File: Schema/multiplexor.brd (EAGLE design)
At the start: 100 x 80 mm, 23 parts, among them IC1 4051D, IC2 4051D, IC3 74LS595N

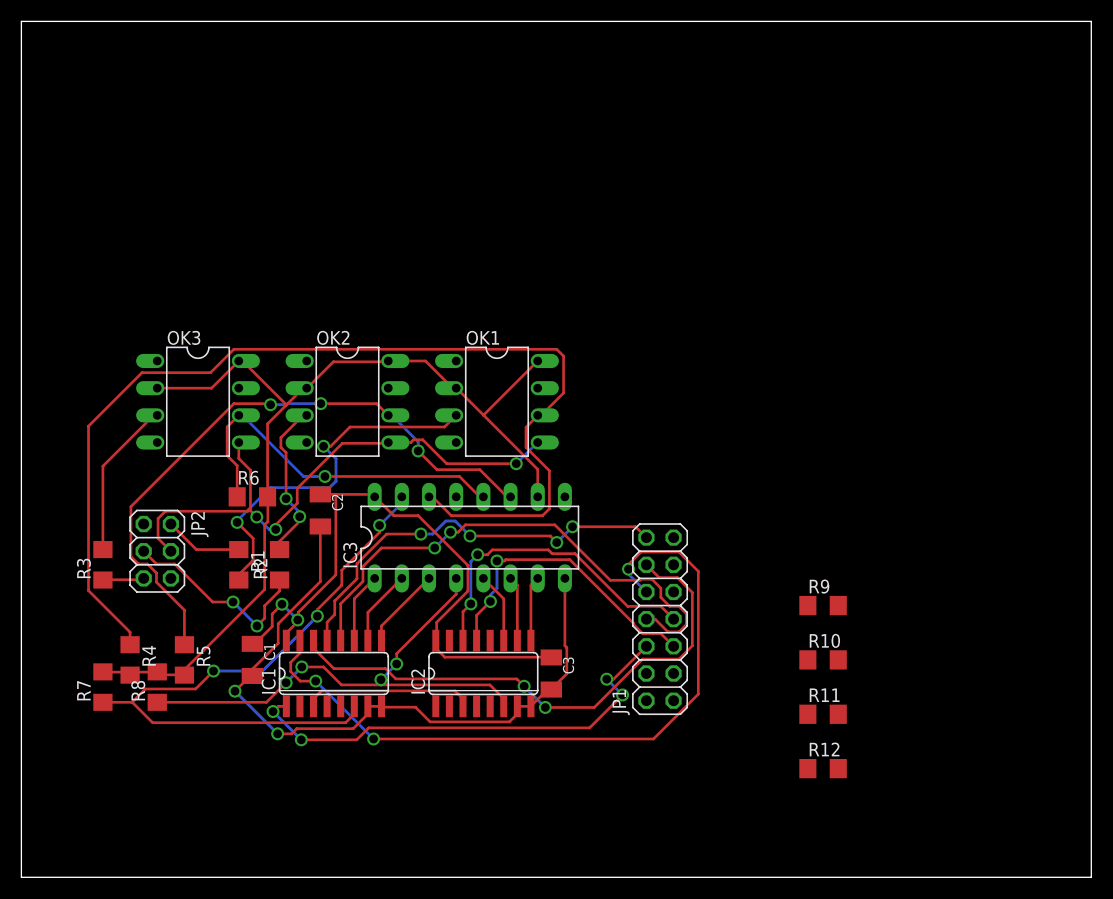
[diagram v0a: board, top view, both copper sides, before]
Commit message: Next release
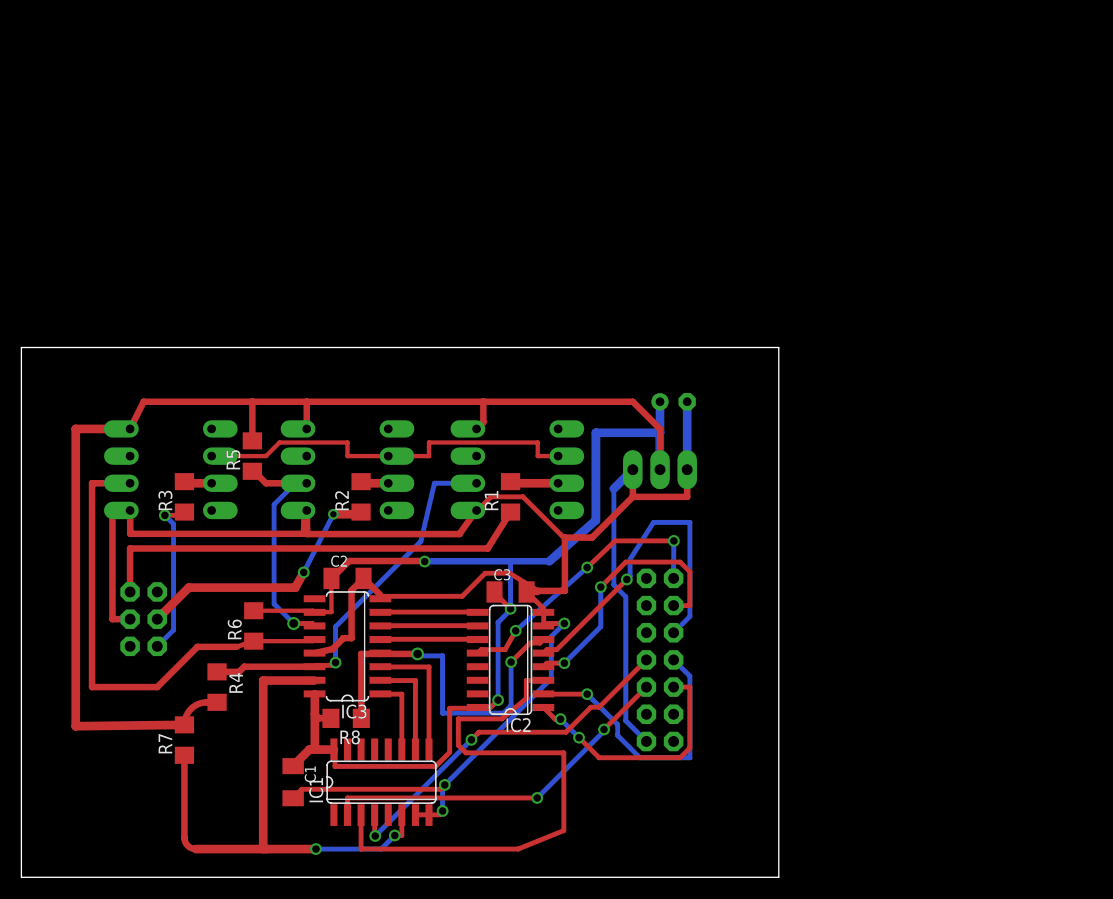
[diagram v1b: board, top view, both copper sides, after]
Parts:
- removed R10, R11, R12, R9: (no value), resistor:R1206
- added C4: (no value), rcl:E2,5-6
- added JP3: (no value), pinhead:1X03
- IC3: value 74LS595N -> 74HC595D; device 74xx-eu:DIL16 -> 74xx-eu:SO16
- moved R1 26.2 mm to (45.7, 35.6), turned to 90 degrees
- moved R5 20.1 mm to (21.6, 39.4), turned to 90 degrees
- moved R8 17.9 mm to (30.4, 14.9), turned to 180 degrees
- moved IC3 15.3 mm to (30.5, 21.6), turned to 90 degrees
- moved R6 12.1 mm to (21.7, 23.5), turned to 90 degrees
- moved C1 12.0 mm to (25.4, 8.89)
- moved IC1 11.1 mm to (33.7, 8.89)
- moved R2 9.92 mm to (31.8, 35.6)
- moved R3 9.92 mm to (15.2, 35.6)
- moved R7 9.09 mm to (15.2, 12.8)
- moved C3 8.52 mm to (45.7, 26.7), turned to 0 degrees
- moved R4 8.52 mm to (18.3, 17.8)
- moved OK3 6.84 mm to (14.0, 38.1), flipped to the bottom
- moved C2 6.84 mm to (30.5, 27.9), turned to 0 degrees
- moved OK1 6.63 mm to (46.4, 38.1), flipped to the bottom
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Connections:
- removed net +6V: IC3.10, OK1.2, OK1.8, OK2.2, OK2.8, OK3.2, OK3.8, R4.2, R5.2, R6.2, R7.2, R8.2
- removed net N$27: C1.2, C2.2, C3.2, IC1.7, IC1.8, IC2.7, IC2.8, IC3.8
- net +5V: now also OK1.2, OK2.2, OK3.2
- net GND: no longer OK1.5, OK2.5, OK3.5
- net GNDA: now also C1.2, C2.2, C3.2, C4.-, IC1.7, IC1.8, IC2.7, IC2.8, IC3.8, JP1.14, JP3.1, JP3.3, OK1.5, OK2.5, OK3.5
- net N$10: now also IC1.2, JP1.10; no longer IC1.13, JP1.14
- net N$11: now also IC2.12, JP1.1; no longer IC1.14, JP1.12
- net N$12: now also IC1.4, JP1.8; no longer IC1.15, JP1.10
- net N$13: now also IC2.4, JP1.3; no longer IC1.12, JP1.8
- net N$14: now also IC2.5, JP1.5; no longer IC1.1, JP1.6
- net N$15: now also IC2.2, JP1.7; no longer IC2.13, JP1.5
- net N$16: now also IC2.1, JP1.9; no longer IC2.14, JP1.7
- net VCC: now also C4.+, IC3.10, JP3.2, OK1.8, OK2.8, OK3.8, R4.2, R5.2, R6.2, R7.2, R8.2
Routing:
- net GNDA: track 0.00 -> 185.3 mm, vias 0 -> 3
- net VCC: track 59.3 -> 218.8 mm, vias 2 -> 3
- net +6V: track 91.4 -> 0.00 mm
- net N$27: track 64.8 -> 0.00 mm, vias 2 -> 0
- net N$20: track 98.7 -> 35.6 mm, vias 0 -> 1
- net GND: track 53.2 -> 11.8 mm, vias 3 -> 0
- net +5V: track 0.00 -> 36.7 mm
- net N$9: track 16.0 -> 52.7 mm
- net N$21: track 59.2 -> 23.3 mm, vias 3 -> 1
- net N$23: track 7.34 -> 41.5 mm
- net N$12: track 68.2 -> 34.2 mm, vias 3 -> 2
- net N$17: track 34.8 -> 4.54 mm, vias 2 -> 0
- net N$11: track 51.1 -> 26.2 mm, vias 2 -> 3
- net N$13: track 49.2 -> 25.0 mm
- net N$5: track 48.6 -> 34.1 mm, vias 4 -> 2
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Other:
- board size 100 x 80 mm -> 70.8 x 49.5 mm
